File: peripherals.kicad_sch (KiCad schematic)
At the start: 0 parts

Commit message: components selection
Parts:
- added C2, C3: 100n 50V, Capacitor_SMD:C_0603_1608Metric, symbol Device:C_Small
- added R1: 47k 1%, Resistor_SMD:R_0603_1608Metric, symbol Device:R_Small
- added U10: AT30TS75A-XM8M-T, Package_SO:MSOP-8_3x3mm_P0.65mm, symbol Sensor_Temperature:MCP9808_MSOP
- added U11: M24256-BR (MB85RC16V), Package_SO:SOIC-8_3.9x4.9mm_P1.27mm, symbol M24256-BR:M24256-BR
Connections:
- new net: R1.2, U10.3 (Alert)
- new net +3V3: C2.2, C3.1, R1.1, U10.8 (VDD), U11.8 (VCC)
- new net GND: C2.1, C3.2, U10.4 (GND), U10.5 (A2), U10.6 (A1), U10.7 (A0), U11.1 (E0), U11.2 (E1), U11.3 (E2), U11.4 (VSS)
- new net MEM_WC: U11.7 (~{WC})
- new net SCL: U10.2 (SCL), U11.6 (SCL)
- new net SDA: U10.1 (SDA), U11.5 (SDA)

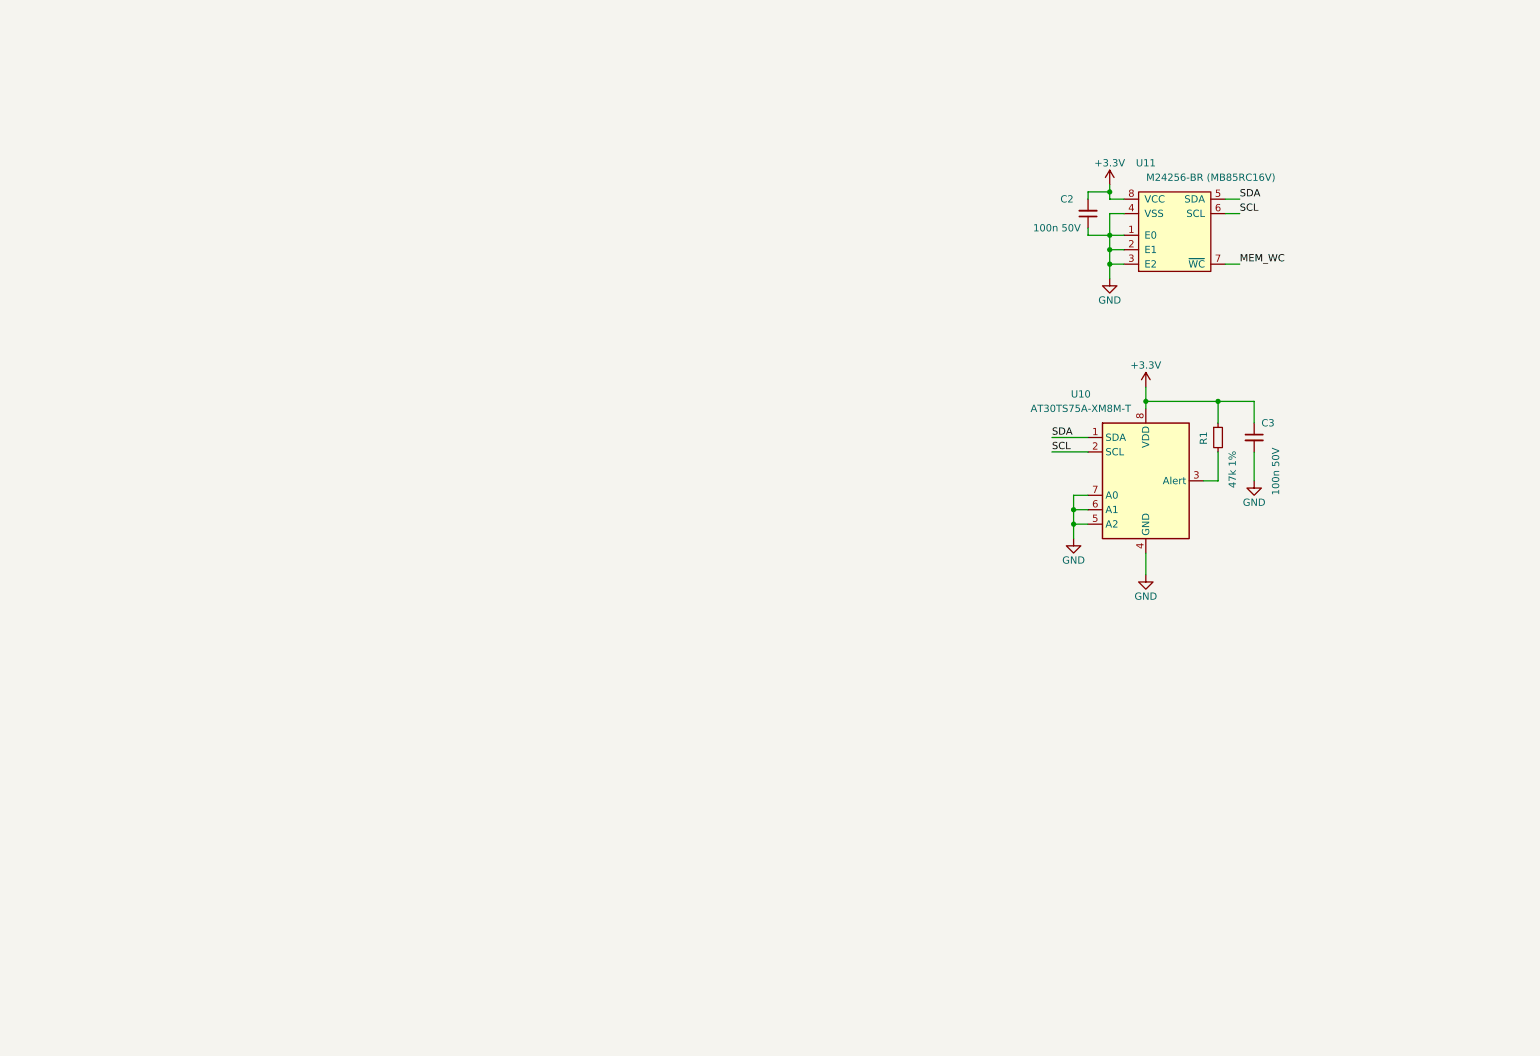
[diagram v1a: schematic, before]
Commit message: Schematic in progress
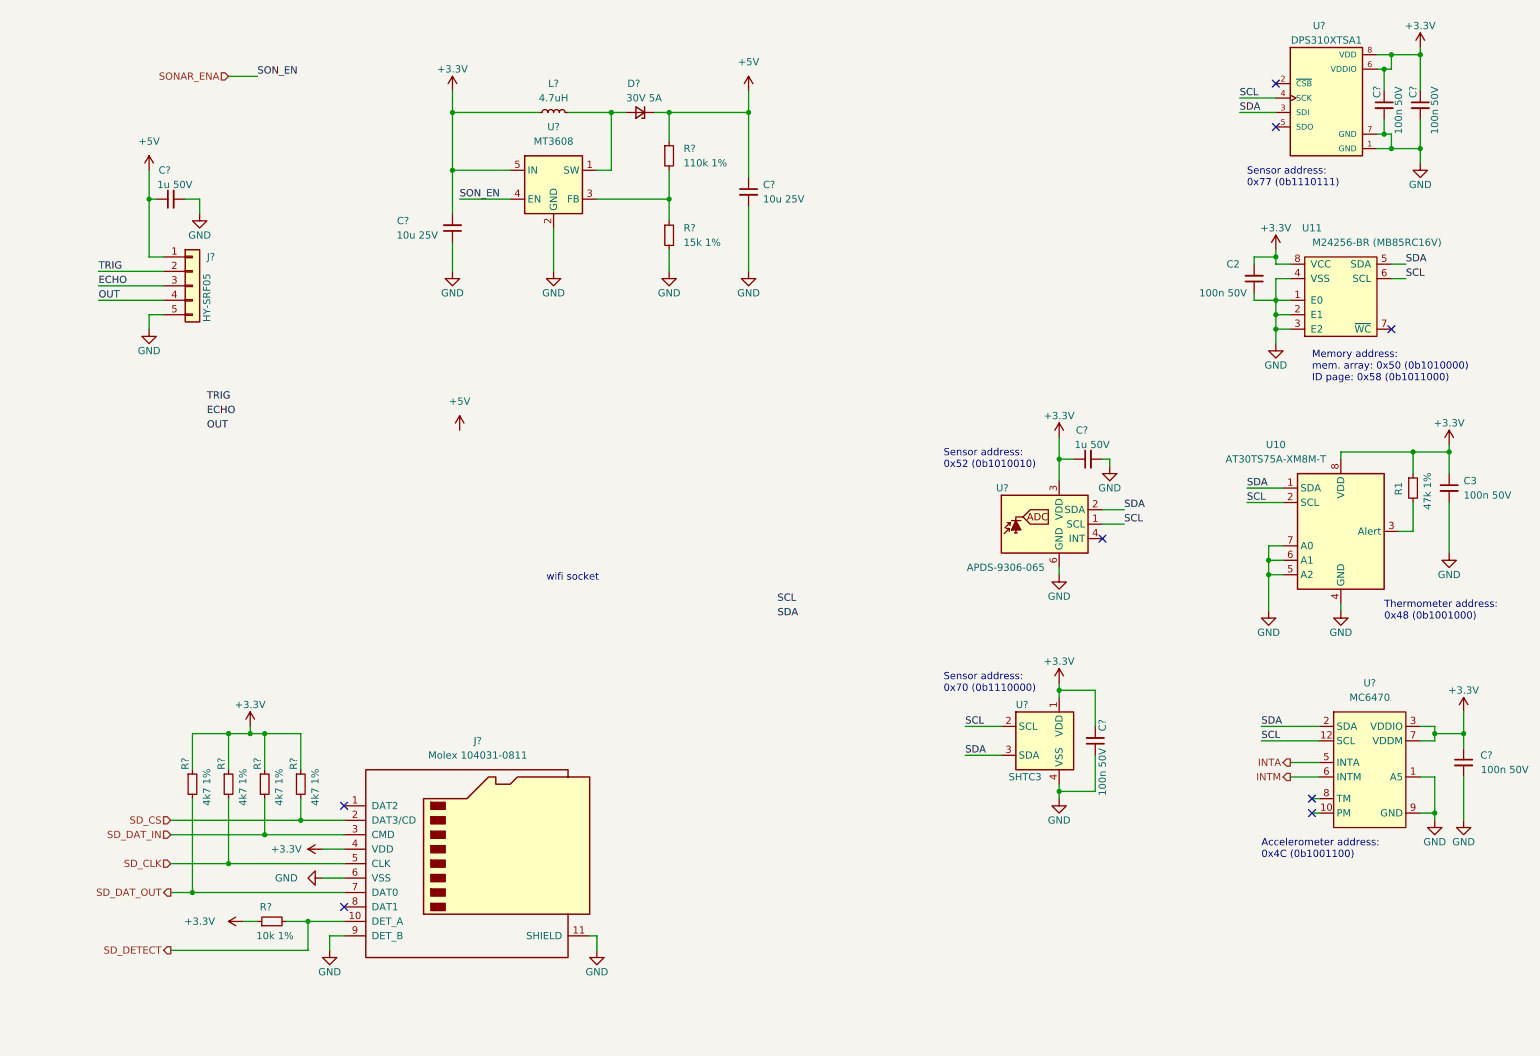
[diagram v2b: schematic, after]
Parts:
- added C? (x2): 10u 25V, Capacitor_SMD:C_0805_2012Metric, symbol Device:C_Small
- added C? (x3): 100n 50V, Capacitor_SMD:C_0603_1608Metric, symbol Device:C_Small
- added C? (x2): 1u 50V, Capacitor_SMD:C_0603_1608Metric, symbol Device:C_Small
- added C?: 100n 50V, Capacitor_SMD:C_0603_1608Metric_Pad1.08x0.95mm_HandSolder, symbol Device:C_Small
- added D?: 30V 5A, Diode_SMD:D_SOD-128, symbol Device:D_Zener_Small
- added J?: Molex 104031-0811, Connector_Card:microSD_HC_Molex_104031-0811, symbol Connector:Micro_SD_Card_Det
- added J?: HY-SRF05, Connector_PinSocket_2.54mm:PinSocket_1x05_P2.54mm_Vertical, symbol Connector_Generic:Conn_01x05
- added L?: 4.7uH, Inductor_SMD:L_Wuerth_MAPI-3020, symbol Device:L_Small
- added R? (x4): 4k7 1%, Resistor_SMD:R_0603_1608Metric, symbol Device:R_Small
- added R?: 10k 1%, Resistor_SMD:R_0603_1608Metric, symbol Device:R_Small
- added R?: 110k 1%, Resistor_SMD:R_0603_1608Metric, symbol Device:R_Small
- added R?: 15k 1%, Resistor_SMD:R_0603_1608Metric, symbol Device:R_Small
- added U?: APDS-9306-065, OptoDevice:Broadcom_DFN-6_2x2mm_P0.65mm, symbol Sensor_Optical:APDS-9306-065
- added U?: MT3608, Package_TO_SOT_SMD:SOT-23-6, symbol Regulator_Switching:MT3608
- added U?: DPS310XTSA1, Package_LGA:Bosch_LGA-8_2x2.5mm_P0.65mm_ClockwisePinNumbering, symbol DPS310XTSA1:DPS310XTSA1
- added U?: MC6470, Package_LGA:LGA-12_2x2mm_P0.5mm, symbol MC6470:MC6470
- added U?: SHTC3, Sensor_Humidity:Sensirion_DFN-4-1EP_2x2mm_P1mm_EP0.7x1.6mm, symbol Sensor_Humidity:SHTC3
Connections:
- net +3V3: now also C?.1, C?.1, C?.1, C?.1, C?.2, C?.2, J?.4 (VDD), L?.1, R?.1, R?.1, R?.1, R?.1, R?.1, U?.1 (VDD), U?.3 (VDD), U?.3 (VDDIO), U?.5 (IN), U?.6 (VDDIO), U?.7 (VDDM), U?.8 (VDD)
- net GND: now also C?.1, C?.1, C?.2, C?.2, C?.2, C?.2, C?.2, C?.2, J?.11 (SHIELD), J?.5 (Pin_5), J?.6 (VSS), J?.9 (DET_B), R?.2, U?.1 (A5), U?.1 (GND), U?.2 (GND), U?.4 (VSS), U?.6 (GND), U?.7 (GND), U?.9 (GND)
- net SCL: now also U?.1 (SCL), U?.12 (SCL), U?.2 (SCL), U?.4 (SCK)
- net SDA: now also U?.2 (SDA), U?.2 (SDA), U?.3 (SDA), U?.3 (SDI)
- net MEM_WC: no longer names the net of U11.7 (~{WC})
- new net: D?.2 (A), L?.2, U?.1 (SW)
- new net: R?.1, R?.2, U?.3 (FB)
- new net +5V: C?.1, C?.1, D?.1 (K), J?.1 (Pin_1), R?.1
- new net ECHO: J?.3 (Pin_3)
- new net INTA: U?.5 (INTA)
- new net INTM: U?.6 (INTM)
- new net OUT: J?.4 (Pin_4)
- new net SD_CLK: J?.5 (CLK), R?.2
- new net SD_CS: J?.2 (DAT3/CD), R?.2
- new net SD_DAT_IN: J?.3 (CMD), R?.2
- new net SD_DAT_OUT: J?.7 (DAT0), R?.2
- new net SD_DETECT: J?.10 (DET_A), R?.2
- new net SONAR_ENA: U?.4 (EN)
- new net TRIG: J?.2 (Pin_2)
- no-connect marks 0 -> 8
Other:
- note added: "Accelerometer address: 0x4C (0b1001100)"
- note added: "Memory address: mem. array: 0x50 (0b1010000) ID page: 0x58 (0b1011000)"
- note added: "Sensor address: 0x52 (0b1010010)"
- note added: "Sensor address: 0x70 (0b1110000)"
- note added: "Sensor address: 0x77 (0b1110111)"
- note added: "Thermometer address: 0x48 (0b1001000)"
- note added: "wifi socket"
- moved on the sheet: C2, C3, R1, U10, U11

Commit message: schematic almost done
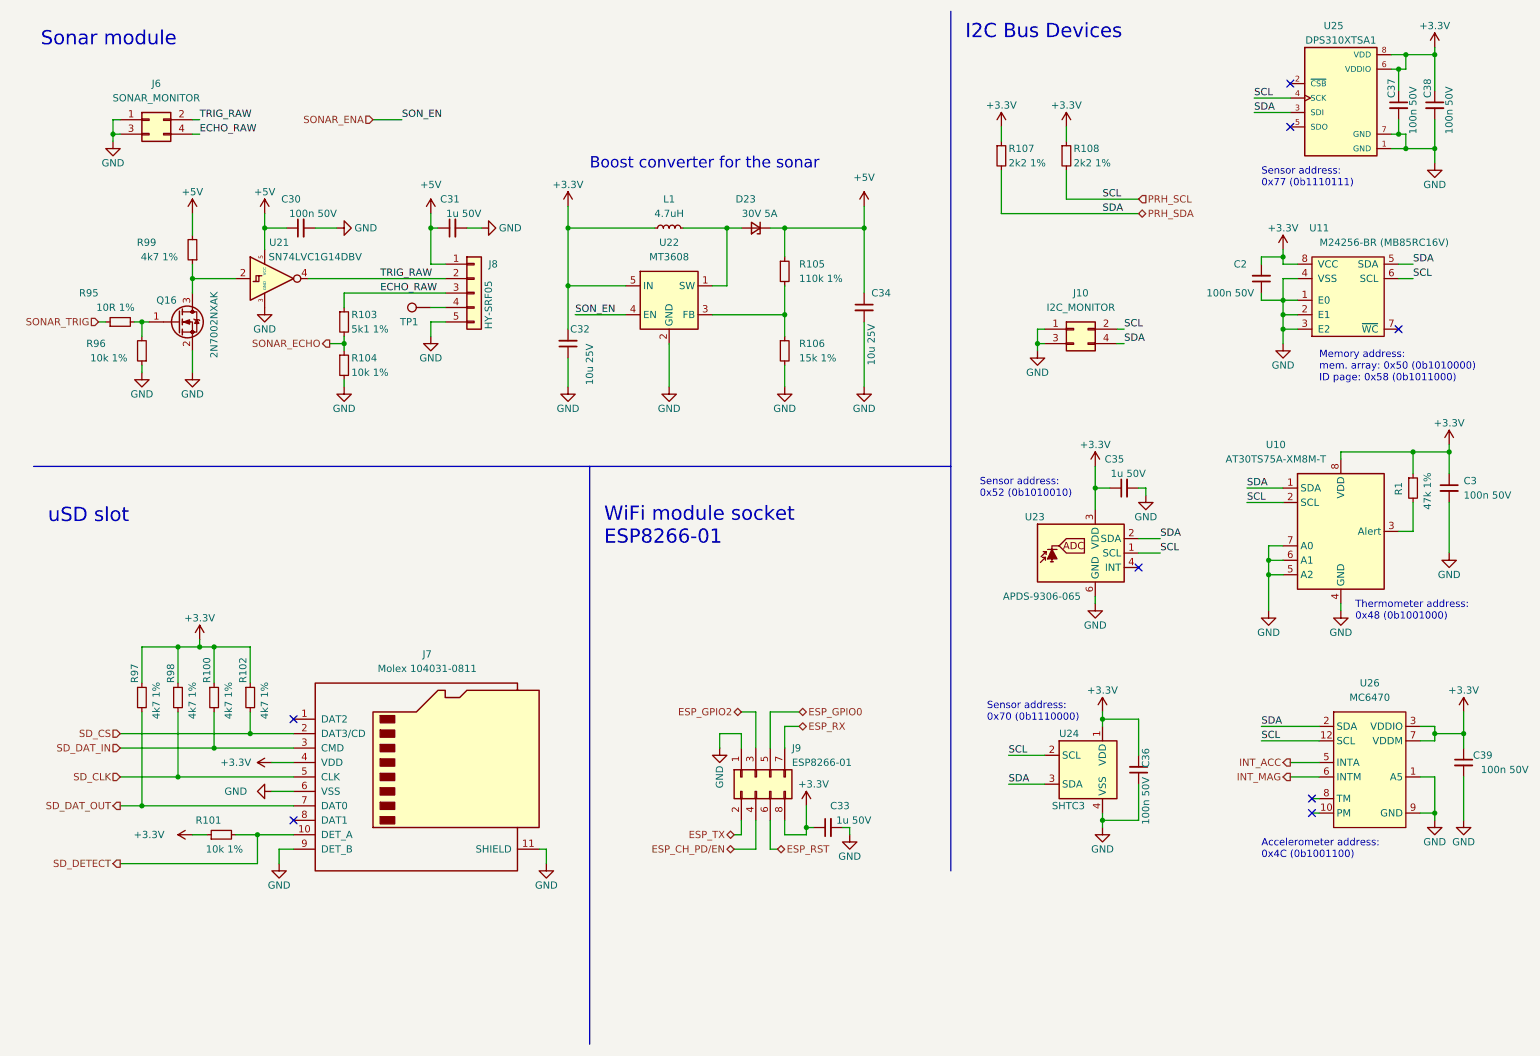
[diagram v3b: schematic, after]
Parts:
- added C30: 100n 50V, Capacitor_SMD:C_0603_1608Metric, symbol Device:C_Small
- added C33: 1u 50V, Capacitor_SMD:C_0603_1608Metric, symbol Device:C_Small
- added J10: I2C_MONITOR, Connector_PinHeader_2.54mm:PinHeader_2x02_P2.54mm_Vertical, symbol Connector_Generic:Conn_02x02_Odd_Even
- added J6: SONAR_MONITOR, Connector_PinHeader_2.54mm:PinHeader_2x02_P2.54mm_Vertical, symbol Connector_Generic:Conn_02x02_Odd_Even
- added J9: ESP8266-01, Connector_PinSocket_2.54mm:PinSocket_2x04_P2.54mm_Vertical, symbol Connector_Generic:Conn_02x04_Odd_Even
- added Q16: 2N7002NXAK, Package_TO_SOT_SMD:SOT-23, symbol Transistor_FET:2N7002
- added R103: 5k1 1%, Resistor_SMD:R_0603_1608Metric_Pad0.98x0.95mm_HandSolder, symbol Device:R_Small
- added R104: 10k 1%, Resistor_SMD:R_0603_1608Metric, symbol Device:R_Small
- added R107, R108: 2k2 1%, Resistor_SMD:R_0603_1608Metric, symbol Device:R_Small
- added R95: 10R 1%, Resistor_SMD:R_0805_2012Metric, symbol Device:R_Small
- added R96: 10k 1%, Resistor_SMD:R_0603_1608Metric_Pad0.98x0.95mm_HandSolder, symbol Device:R_Small
- added R99: 4k7 1%, Resistor_SMD:R_0603_1608Metric_Pad0.98x0.95mm_HandSolder, symbol Device:R_Small
- added TP1: TestPoint, TestPoint:TestPoint_THTPad_D2.5mm_Drill1.2mm, symbol Connector:TestPoint
- added U21: SN74LVC1G14DBV, Package_TO_SOT_SMD:SOT-23-5, symbol 74xGxx:SN74LVC1G14DBV
- gave numbers to parts that had none: 24
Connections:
- net +3V3: now also C33.1, J9.8 (Pin_8), R107.1, R108.1
- net +5V: now also C30.1, R99.2, U21.5 (VCC)
- net GND: now also C30.2, C33.2, J10.1 (Pin_1), J10.3 (Pin_3), J6.1 (Pin_1), J6.3 (Pin_3), J9.1 (Pin_1), Q16.2 (S), R104.2, R96.1, U21.3 (GND)
- net ECHO renamed ECHO_RAW
- net ECHO_RAW: now also J6.4 (Pin_4), R103.1
- net INTA renamed INT_ACC
- net INTM renamed INT_MAG
- net OUT: no longer names the net of J8.4 (Pin_4)
- net OUT: now also TP1.1
- net SCL renamed PRH_SCL
- net PRH_SCL: now also J10.2 (Pin_2), R108.2
- net SDA renamed PRH_SDA
- net PRH_SDA: now also J10.4 (Pin_4), R107.2
- net TRIG renamed TRIG_RAW
- net TRIG_RAW: now also J6.2 (Pin_2), U21.4
- new net: Q16.1 (G), R95.2, R96.2
- new net: Q16.3 (D), R99.1, U21.2
- new net ESP_CH_PD/EN: J9.4 (Pin_4)
- new net ESP_GPIO0: J9.5 (Pin_5)
- new net ESP_GPIO2: J9.3 (Pin_3)
- new net ESP_RST: J9.6 (Pin_6)
- new net ESP_RX: J9.7 (Pin_7)
- new net ESP_TX: J9.2 (Pin_2)
- new net SONAR_ECHO: R103.2, R104.1
- new net SONAR_TRIG: R95.1
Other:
- note added: "Boost converter for the sonar"
- note added: "I2C Bus Devices"
- note added: "Sonar module"
- note added: "WiFi module socket ESP8266-01"
- note added: "uSD slot"
- note removed: "wifi socket"
- moved on the sheet: C2, C31, C32, C34, C35, C36, C37, C38, D23, J7, J8, L1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

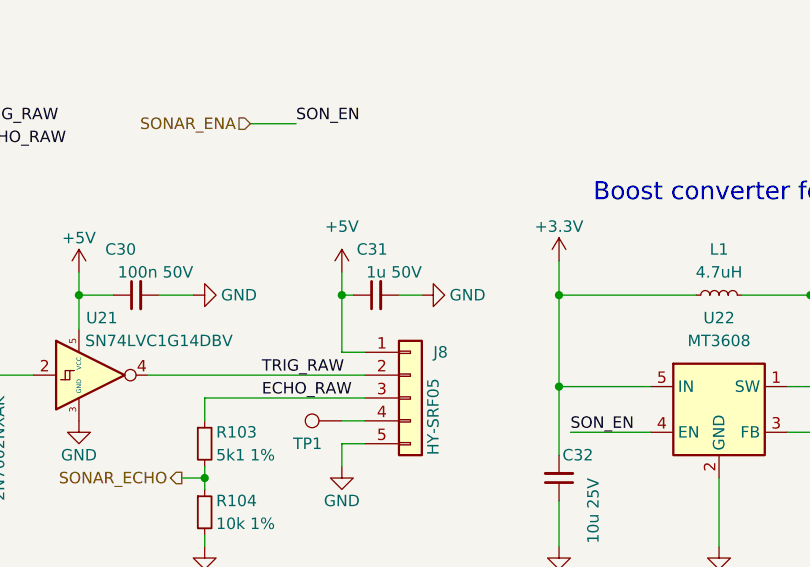
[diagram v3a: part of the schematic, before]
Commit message: layout in progress
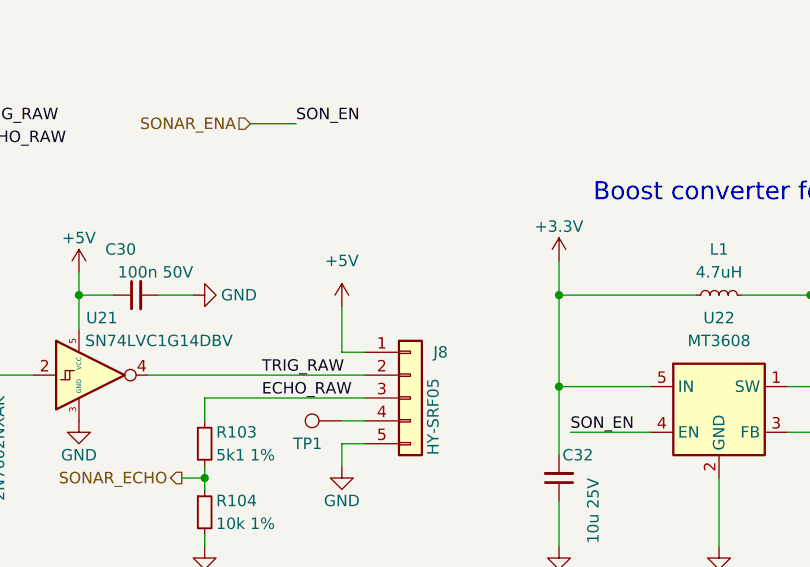
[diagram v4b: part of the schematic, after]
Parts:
- removed C31: 1u 50V, Capacitor_SMD:C_0603_1608Metric, symbol Device:C_Small
- R95: footprint Resistor_SMD:R_0805_2012Metric -> Resistor_SMD:R_0603_1608Metric_Pad0.98x0.95mm_HandSolder
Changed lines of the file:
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@@
   (junction (at 34.29 153.67) (diameter 0) (color 0 0 0 0)
-  )
-  (junction (at 85.09 52.07) (diameter 0) (color 0 0 0 0)
   )
   (junction (at 266.7 140.97) (diameter 0) (color 0 0 0 0)
@@
     (stroke (width 0) (type default) (color 0 0 0 0))
   )
-  (wire (pts (xy 91.44 52.07) (xy 93.98 52.07))
-    (stroke (width 0) (type default) (color 0 0 0 0))
-  )
   (wire (pts (xy 34.29 137.16) (xy 34.29 153.67))
     (stroke (width 0) (type default) (color 0 0 0 0))
@@
     (stroke (width 0) (type default) (color 0 0 0 0))
   )
-  (wire (pts (xy 85.09 49.53) (xy 85.09 52.07))
-    (stroke (width 0) (type default) (color 0 0 0 0))
-  )
   (wire (pts (xy 255.27 24.13) (xy 256.54 24.13))
     (stroke (width 0) (type default) (color 0 0 0 0))
@@
     (stroke (width 0) (type default) (color 0 0 0 0))
   )
-  (wire (pts (xy 85.09 52.07) (xy 86.36 52.07))
-    (stroke (width 0) (type default) (color 0 0 0 0))
-  )
   (wire (pts (xy 85.09 68.58) (xy 87.63 68.58))
     (stroke (width 0) (type default) (color 0 0 0 0))
@@
     (stroke (width 0) (type default) (color 0 0 0 0))
   )
-  (wire (pts (xy 85.09 52.07) (xy 85.09 58.42))
+  (wire (pts (xy 85.09 53.34) (xy 85.09 58.42))
     (stroke (width 0) (type default) (color 0 0 0 0))
   )
@@
       (effects (font (size 1.27 1.27)) (justify left))
     )
-    (property "Footprint" "Resistor_SMD:R_0805_2012Metric" (id 2) (at 30.48 68.58 0)
+    (property "Footprint" "Resistor_SMD:R_0603_1608Metric_Pad0.98x0.95mm_HandSolder" (id 2) (at 30.48 68.58 0)
       (effects (font (size 1.27 1.27)) hide)
     )
@@
     (pin "1")
   )
-  (symbol (lib_id "power:+5V") (at 85.09 49.53 0) (unit 1)
+  (symbol (lib_id "power:+5V") (at 85.09 53.34 0) (unit 1)
     (in_bom yes) (on_board yes) (fields_autoplaced)
-    (property "Reference" "#PWR0138" (id 0) (at 85.09 53.34 0)
-      (effects (font (size 1.27 1.27)) hide)
-    )
-    (property "Value" "+5V" (id 1) (at 85.09 44.45 0))
-    (property "Footprint" "" (id 2) (at 85.09 49.53 0)
-      (effects (font (size 1.27 1.27)) hide)
-    )
-    (property "Datasheet" "" (id 3) (at 85.09 49.53 0)
+    (property "Reference" "#PWR0138" (id 0) (at 85.09 57.15 0)
+      (effects (font (size 1.27 1.27)) hide)
+    )
+    (property "Value" "+5V" (id 1) (at 85.09 48.26 0))
+    (property "Footprint" "" (id 2) (at 85.09 53.34 0)
+      (effects (font (size 1.27 1.27)) hide)
+    )
+    (property "Datasheet" "" (id 3) (at 85.09 53.34 0)
       (effects (font (size 1.27 1.27)) hide)
     )
@@
     (pin "2")
   )
-  (symbol (lib_id "Device:C_Small") (at 88.9 52.07 90) (unit 1)
-    (in_bom yes) (on_board yes)
-    (property "Reference" "C31" (id 0) (at 90.17 46.99 90)
-      (effects (font (size 1.27 1.27)) (justify left))
-    )
-    (property "Value" "1u 50V" (id 1) (at 93.98 49.53 90)
-      (effects (font (size 1.27 1.27)) (justify left))
-    )
-    (property "Footprint" "Capacitor_SMD:C_0603_1608Metric" (id 2) (at 88.9 52.07 0)
-      (effects (font (size 1.27 1.27)) hide)
-    )
-    (property "Datasheet" "~" (id 3) (at 88.9 52.07 0)
-      (effects (font (size 1.27 1.27)) hide)
-    )
-    (pin "1")
-    (pin "2")
-  )
   (symbol (lib_id "power:+3.3V") (at 234.95 55.88 0) (unit 1)
     (in_bom yes) (on_board yes)
@@
       (effects (font (size 1.27 1.27)) hide)
     )
-    (pin "1")
-  )
-  (symbol (lib_id "power:GND") (at 93.98 52.07 90) (unit 1)
-    (in_bom yes) (on_board yes)
-    (property "Reference" "#PWR0140" (id 0) (at 100.33 52.07 0)
-      (effects (font (size 1.27 1.27)) hide)
-    )
-    (property "Value" "GND" (id 1) (at 99.06 52.07 90))
-    (property "Footprint" "" (id 2) (at 93.98 52.07 0)
-      (effects (font (size 1.27 1.27)) hide)
-    )
-    (property "Datasheet" "" (id 3) (at 93.98 52.07 0)
-      (effects (font (size 1.27 1.27)) hide)
-    )

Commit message: schematics update
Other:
- company: (none) -> Wrocław University of Science and Technology
- title: (none) -> Peripherals
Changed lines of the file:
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@@
 (kicad_sch (version 20211123) (generator eeschema)
   (paper "A4")
+  (title_block
+    (title "Peripherals")
+    (date "2023-04-04")
+    (rev "1")
+    (company "Wrocław University of Science and Technology")
+    (comment 1 "Opensource educational robotic platform")
+    (comment 2 "Author: Jakub Mnich (jakub.mnich@pwr.edu.pl)")
+  )
   (junction (at 234.95 64.77) (diameter 0) (color 0 0 0 0)
   )
